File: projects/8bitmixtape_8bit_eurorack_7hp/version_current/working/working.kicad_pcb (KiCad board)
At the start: 2 copper layers, 33.3 x 106.7 mm, 51 parts, among them J1 CONN_01X04, J2 CONN_01X04, J4 Con_3-5V, J5 Conn_01x02, J6 Sync_Jumper, J7 Conn_02x05_Odd_Even, J8 Conn_01x02, J9 Sync_Jumper, SW2 SW_Push, SW3 SW_Push, SW4 SW_Push, U1 ATTINY85-20SU, U3 7805

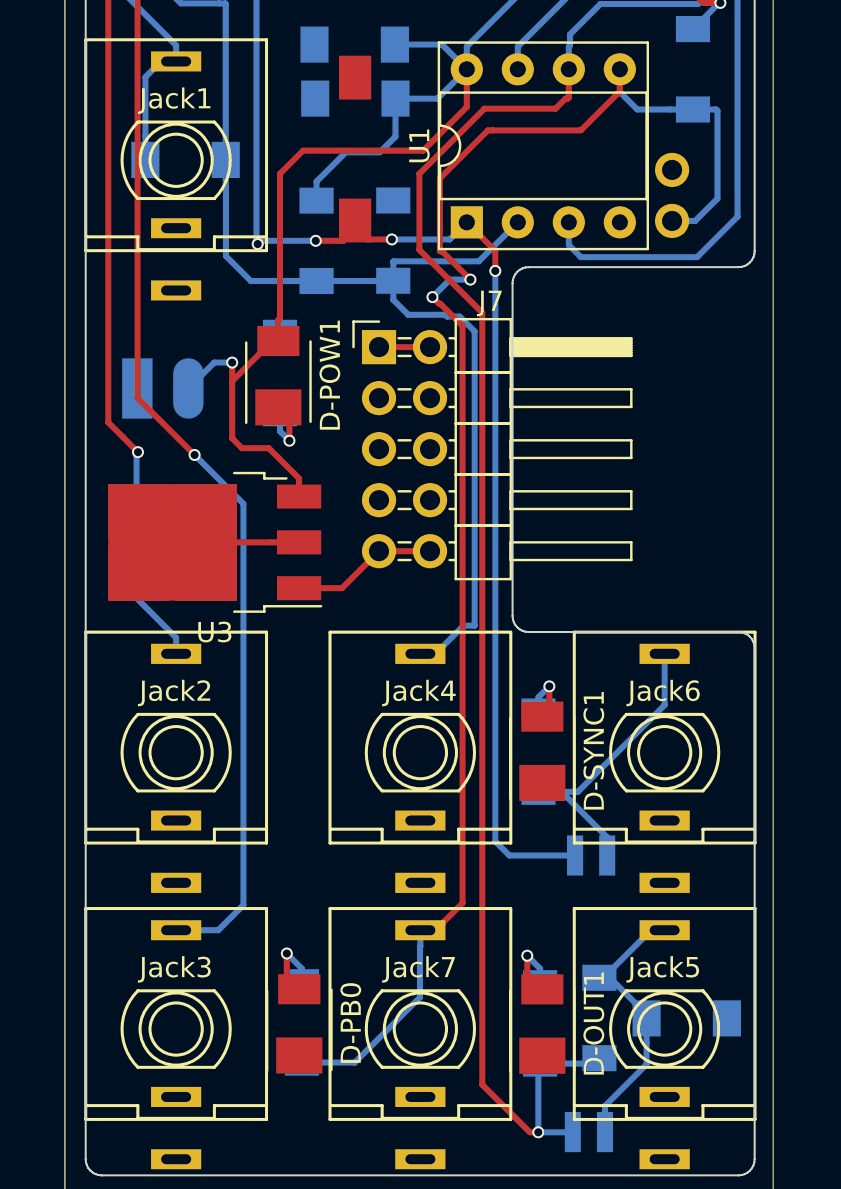
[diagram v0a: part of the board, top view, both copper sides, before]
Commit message: updated all projects from src
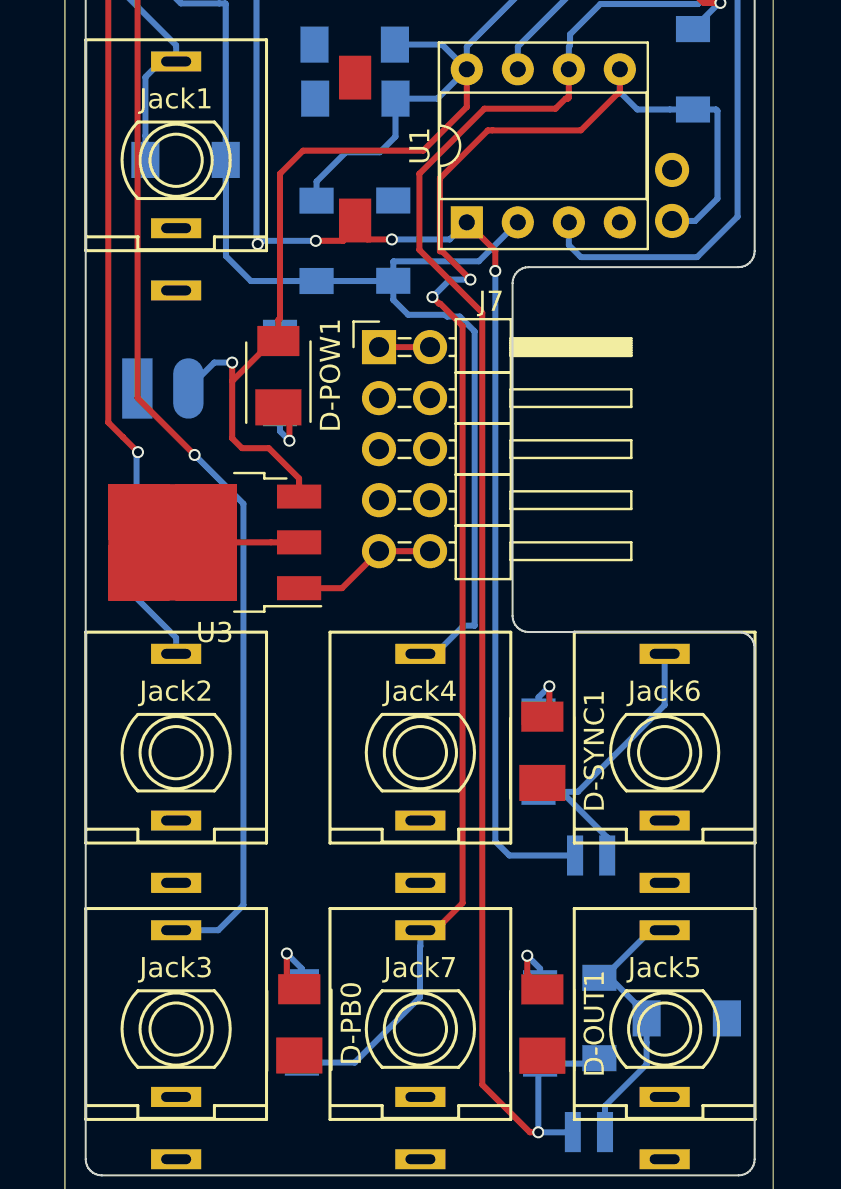
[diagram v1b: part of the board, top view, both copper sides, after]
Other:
- net class Default added: clearance 0.3, trace_width 0.3, via_dia 0.6, via_drill 0.4
- net class thinSiech added: clearance 0.2, trace_width 0.3, via_dia 0.6, via_drill 0.4
